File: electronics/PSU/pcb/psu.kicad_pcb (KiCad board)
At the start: 2 copper layers, 73 x 80 mm, 132 parts, among them J1 Conn_01x02_Socket, J2 Conn_01x02_Socket, J3 Conn_01x02_Socket, J4 Conn_01x02_Socket, J5 Conn_01x02_Socket, J6 Conn_01x02_Socket, J7 Conn_01x02_Socket, J8 Conn_01x02_Socket, U1 ADPL16000B, U2 LTC3260xDE, U3 ADPL54203, U4 ADPL54203

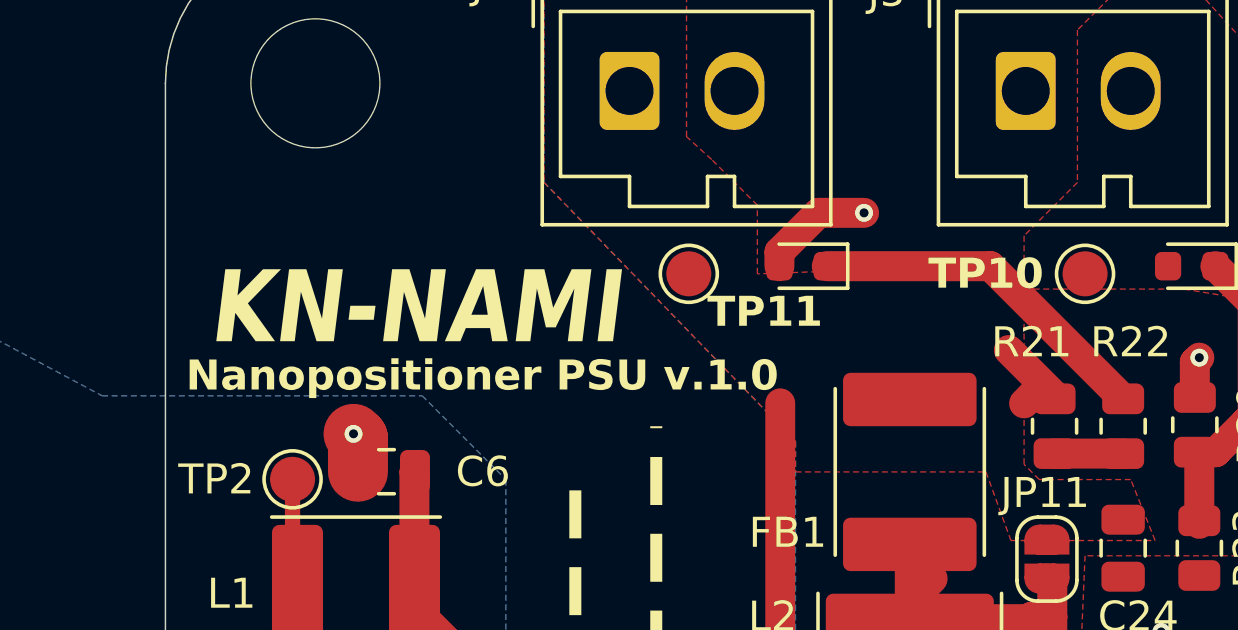
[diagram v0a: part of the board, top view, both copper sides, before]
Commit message: update pcb signature
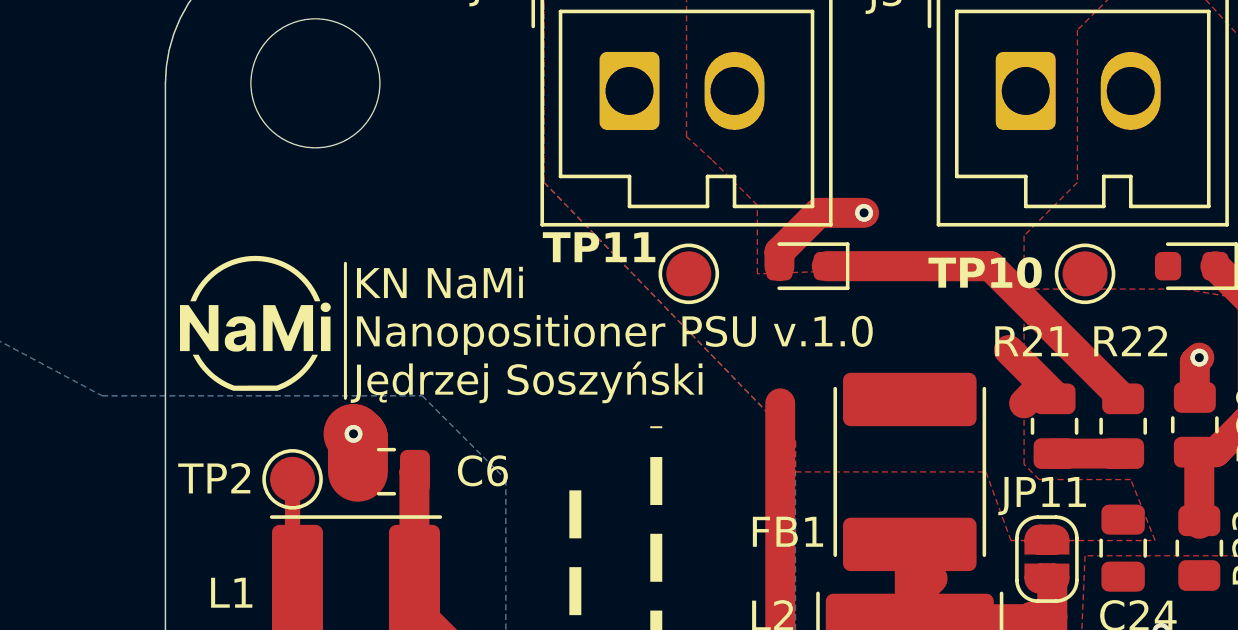
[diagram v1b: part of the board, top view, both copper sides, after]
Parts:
- added G***: LOGO, Symbol:nami_logo_4.5mm, F.Cu at (-2.00, 8.00)
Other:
- board text added: "KN NaMi Nanopositioner PSU v.1.0 Jędrzej Soszyński"
- board text removed: "KN-NAMI"
- board text removed: "Nanopositioner PSU v.1.0"
